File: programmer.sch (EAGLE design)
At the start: 20 parts, among them IC1 74ABT125DB, U1 ATMEGA8U2, X1 16MHz

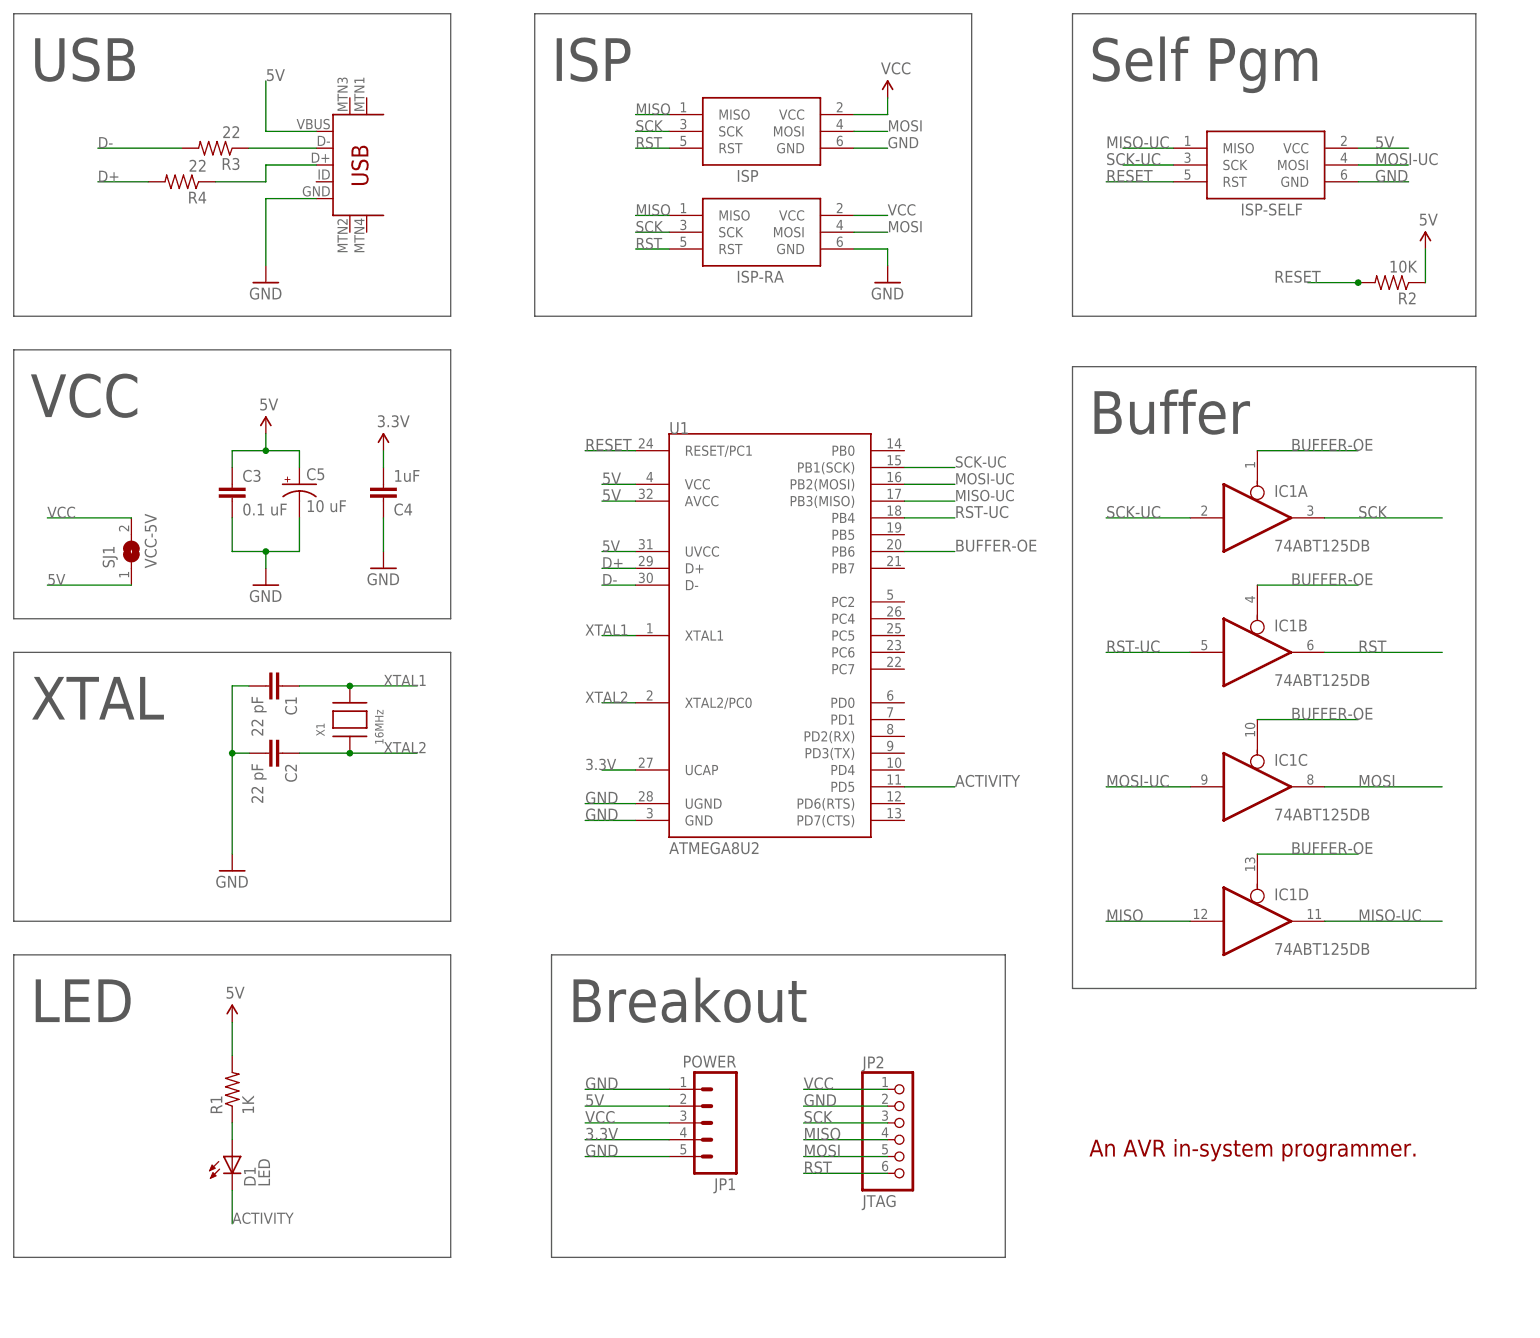
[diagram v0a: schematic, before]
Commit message: Everything is messed up.
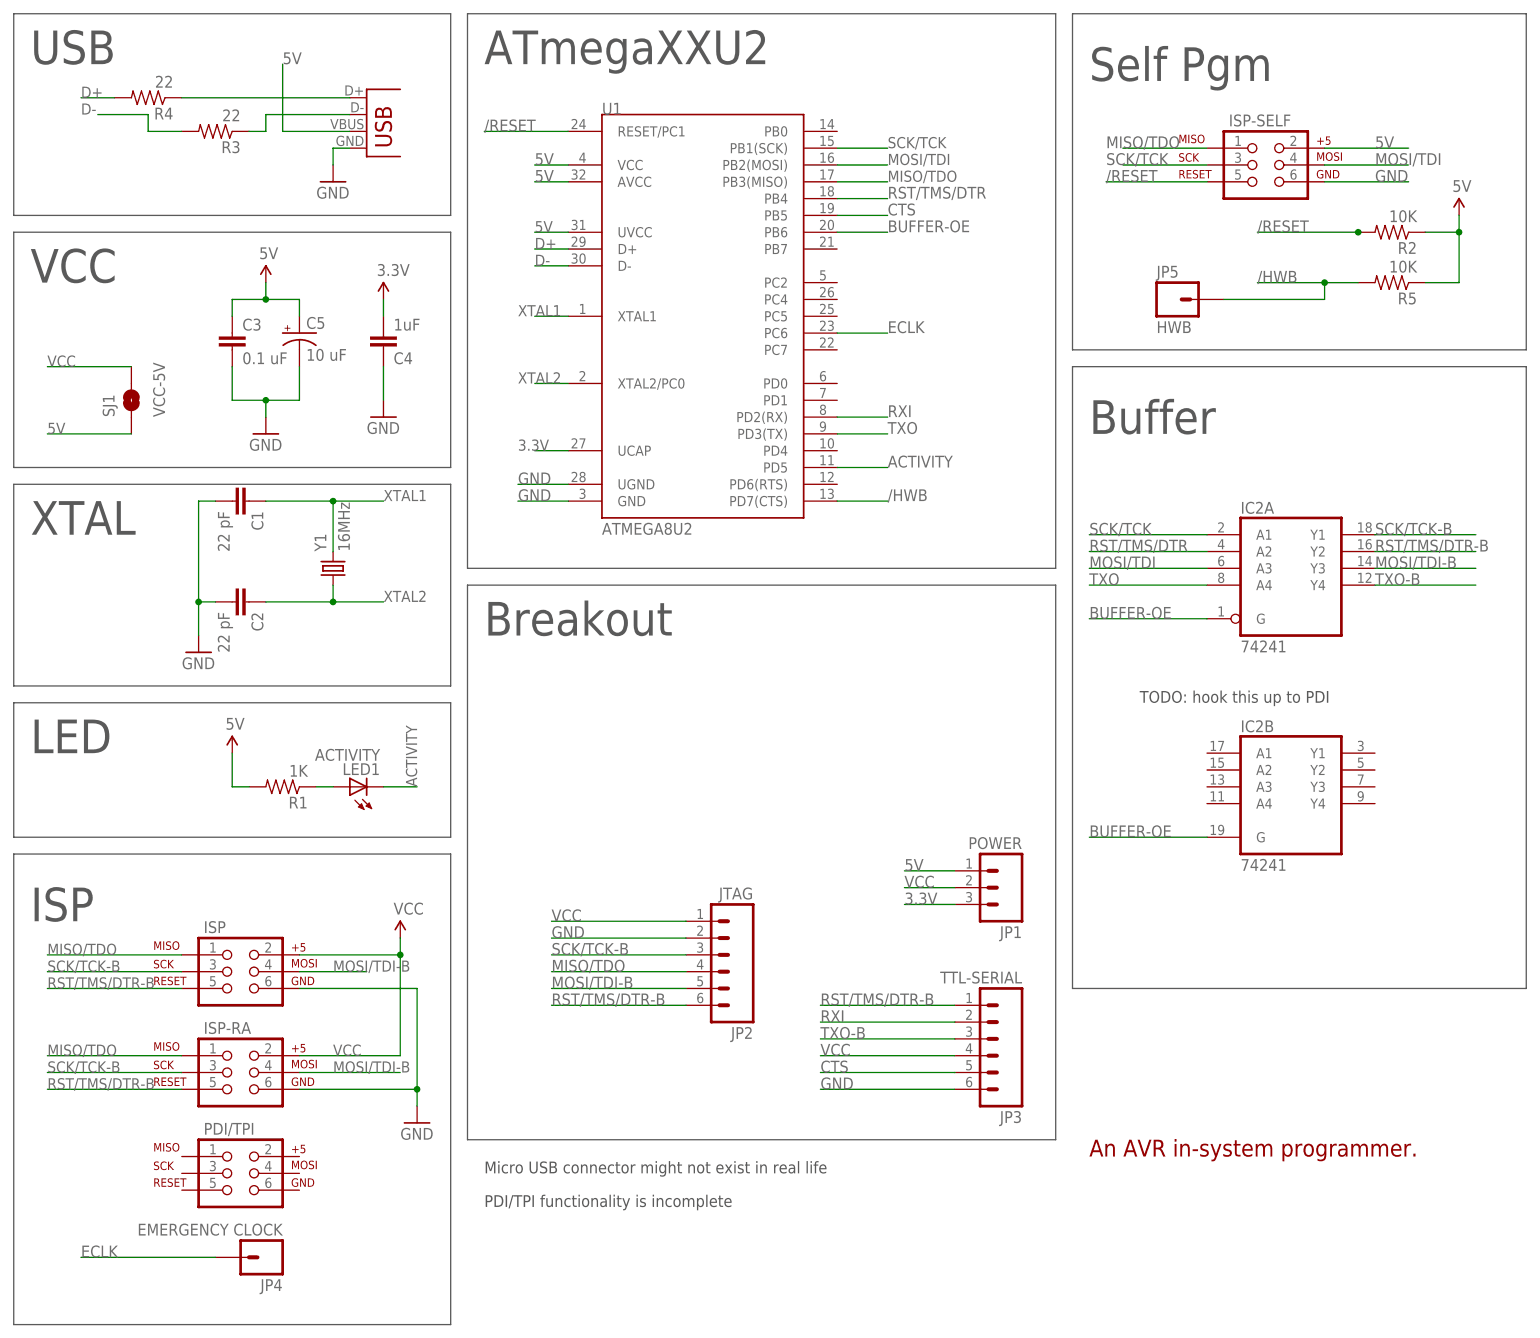
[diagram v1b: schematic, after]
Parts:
- removed D1: LED, adafruit:LEDSMT1206
- removed IC1: 74ABT125DB, 74xx-us:74ABT125DB
- removed USB: USB-MINIB-5PIN, SparkFun:USB-MINIB-5PIN
- removed X1: 16MHz, adafruit:XTALNX8045
- added IC2: 74241, programmer:74241
- added JP3: TTL-SERIAL, SparkFun:M06LOCK
- added JP4: EMERGENCY CLOCK, SparkFun:M01PTH
- added JP5: HWB, SparkFun:M01PTH
- added LED1: ACTIVITY, programmer:SPARKFUN_LED
- added PDI/TPI: AVR_SPI_PRG_62X3_LOCK, SparkFun:AVR_SPI_PRG_62X3_LOCK
- added R5: 10K, SparkFun:RESISTOR0805-RES
- added X2: USB-MICROB, SparkFun:USB-MICROB
- added Y1: 16MHz, SparkFun:CRYSTAL5X3
- ISP, ISP-RA, ISP-SELF: value AVRISP-6 -> AVR_SPI_PRG_62X3_LOCK; device adafruit:AVRISP-6 -> SparkFun:AVR_SPI_PRG_62X3_LOCK
- JP1: device SparkFun:M05PTH -> SparkFun:M03LOCK
- JP2: device adafruit:PINHD-1X6 -> SparkFun:M06LOCK
- SJ1: device jumper:SJ -> SparkFun:SOLDERJUMPERNC
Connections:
- removed net MISO: IC1D.I, ISP-RA.MISO, ISP.MISO, JP2.4
- removed net MISO-UC: IC1D.O, ISP-SELF.MISO, U1.PB3(MISO)
- removed net MOSI: IC1C.O, ISP-RA.MOSI, ISP.MOSI, JP2.5
- removed net MOSI-UC: IC1C.I, ISP-SELF.MOSI, U1.PB2(MOSI)
- removed net RESET: ISP-SELF.RST, R2.2, U1.RESET/PC1
- removed net RST: IC1B.O, ISP-RA.RST, ISP.RST, JP2.6
- removed net RST-UC: IC1B.I, U1.PB4
- removed net SCK: IC1A.O, ISP-RA.SCK, ISP.SCK, JP2.3
- removed net SCK-UC: IC1A.I, ISP-SELF.SCK, U1.PB1(SCK)
- new net /HWB: JP5.1, R5.2, U1.PD7(CTS)
- new net /RESET: ISP-SELF.5, R2.2, U1.RESET/PC1
- new net CTS: JP3.5, U1.PB5
- new net ECLK: JP4.1, U1.PC6
- new net MISO/TDO: ISP-RA.1, ISP-SELF.1, ISP.1, JP2.4, U1.PB3(MISO)
- new net MOSI/TDI: IC2A.A3, ISP-SELF.4, U1.PB2(MOSI)
- new net MOSI/TDI-B: IC2A.Y3, ISP-RA.4, ISP.4, JP2.5
- new net RST/TMS/DTR: IC2A.A2, U1.PB4
- new net RST/TMS/DTR-B: IC2A.Y2, ISP-RA.5, ISP.5, JP2.6, JP3.1
- new net RXI: JP3.2, U1.PD2(RX)
- new net SCK/TCK: IC2A.A1, ISP-SELF.3, U1.PB1(SCK)
- new net SCK/TCK-B: IC2A.Y1, ISP-RA.3, ISP.3, JP2.3
- new net TXO: IC2A.A4, U1.PD3(TX)
- new net TXO-B: IC2A.Y4, JP3.3
- net 3.3V: now also JP1.3; no longer JP1.4
- net 5V: now also ISP-SELF.2, JP1.1, R5.1, X2.VBUS; no longer ISP-SELF.VCC, JP1.2, USB.VBUS
- net ACTIVITY: now also LED1.C; no longer D1.C
- net BUFFER-OE: now also IC2A.G, IC2B.G; no longer IC1A.OE, IC1B.OE, IC1C.OE, IC1D.OE
- net D+RAW: now also X2.D+; no longer USB.D+
- net D-RAW: now also X2.D-; no longer USB.D-
- net GND: now also ISP-RA.6, ISP-SELF.6, ISP.6, JP3.6, X2.GND; no longer ISP-RA.GND, ISP-SELF.GND, ISP.GND, JP1.1, JP1.5, USB.GND
- net VCC: now also ISP-RA.2, ISP.2, JP1.2, JP3.4; no longer ISP-RA.VCC, ISP.VCC, JP1.3
- net VCC-LED: now also LED1.A; no longer D1.A
- net XTAL1: now also Y1.2; no longer X1.P$2
- net XTAL2: now also Y1.1; no longer X1.P$1
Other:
- note added: "ATmegaXXU2"
- note added: "Micro USB connector might not exist in real life"
- note added: "PDI/TPI functionality is incomplete"
- note added: "TODO: hook this up to PDI"
- moved on the sheet: C1, C2, C3, C4, C5, R1, R2, R3, R4, U1
